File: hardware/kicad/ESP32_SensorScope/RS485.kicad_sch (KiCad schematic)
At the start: 27 parts, among them J1 RS485_A, J2 RS485_B, J3 RS485_A, J4 RS485_B, Q1 PMOS, Q2 NMOS, U3 SN74LV1T125DBV, U4 SP3481CN OR SN65HVD485E, U5 ASSR-1218

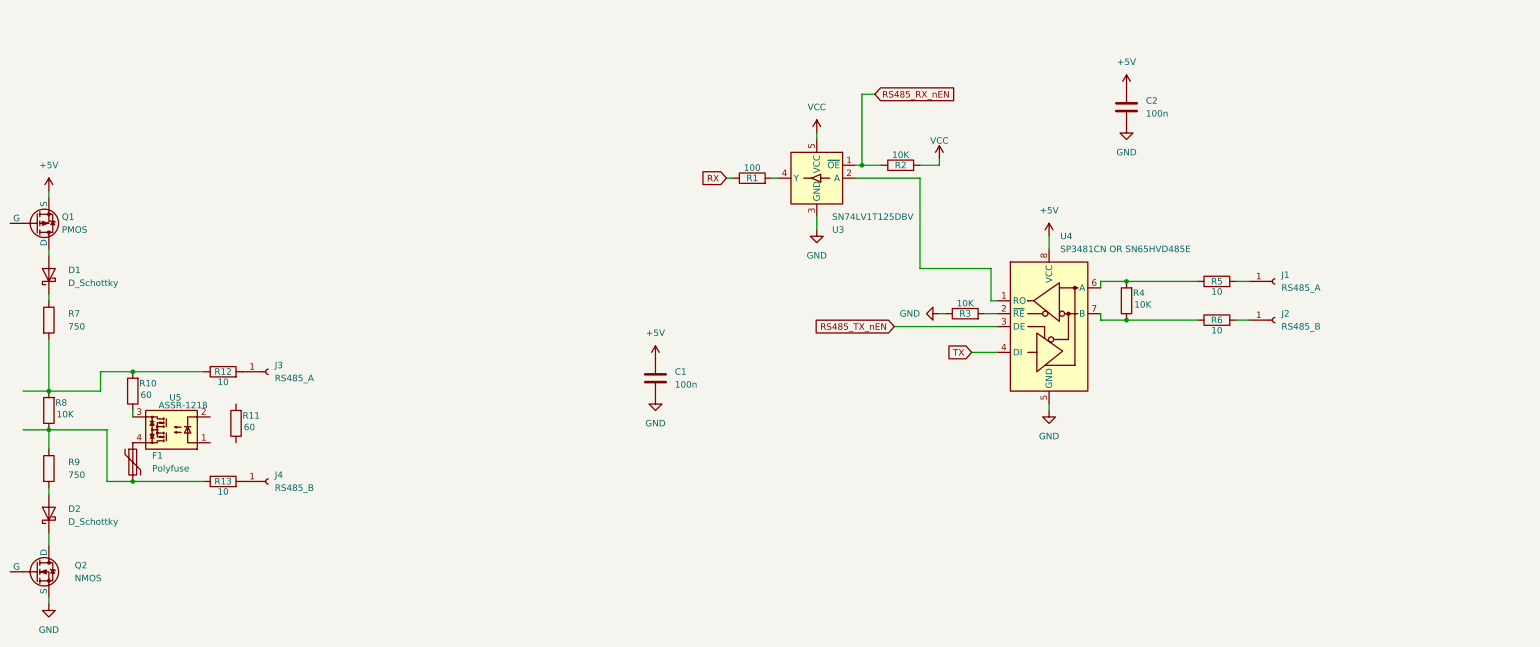
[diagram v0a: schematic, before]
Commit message: Various changes
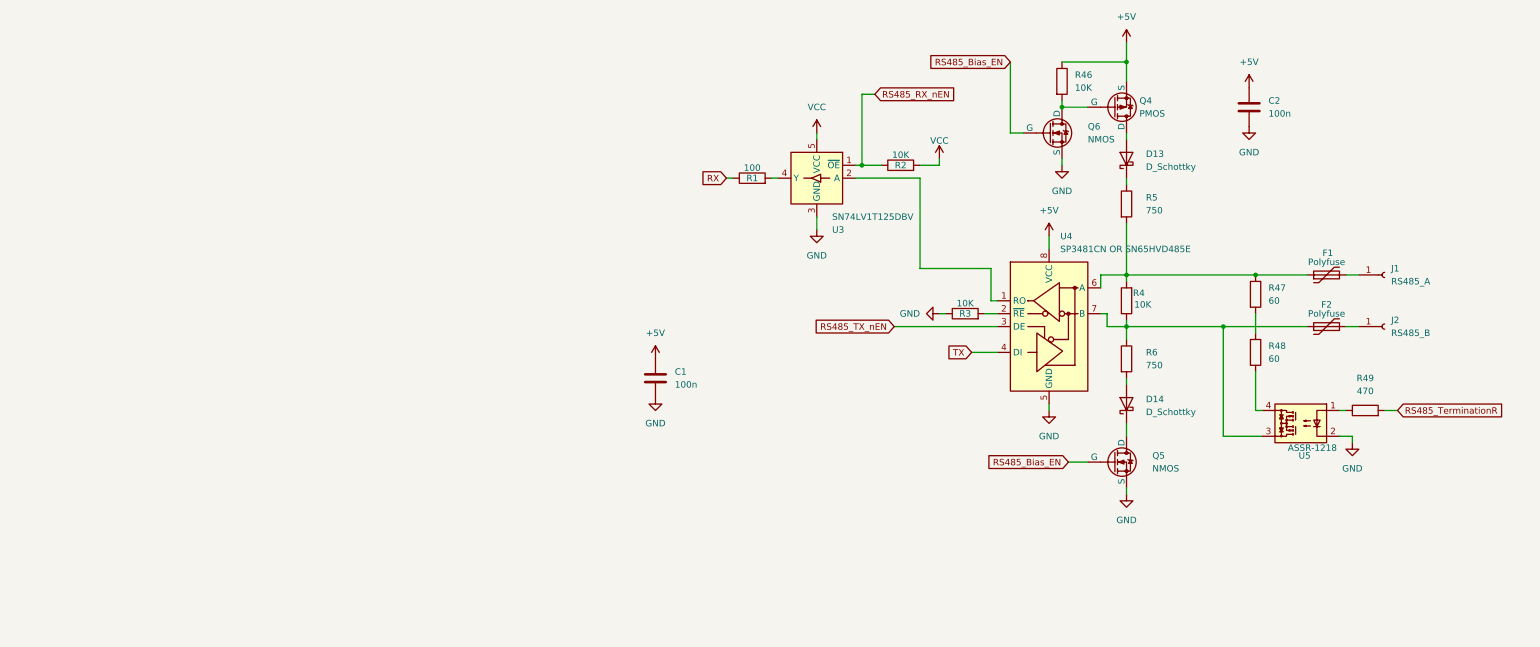
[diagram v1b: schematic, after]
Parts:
- removed D1, D2: D_Schottky, symbol Device:D_Schottky
- removed J3: RS485_A, symbol Connector:Conn_01x01_Socket
- removed J4: RS485_B, symbol Connector:Conn_01x01_Socket
- removed Q1: PMOS, symbol Simulation_SPICE:PMOS
- removed Q2: NMOS, symbol Simulation_SPICE:NMOS
- removed R10, R11: 60, symbol Device:R
- removed R12, R13: 10, symbol Device:R
- removed R7, R9: 750, symbol Device:R
- removed R8: 10K, symbol Device:R
- added D13, D14: D_Schottky, symbol Device:D_Schottky
- added F2: Polyfuse, symbol Device:Polyfuse
- added Q4: PMOS, symbol Simulation_SPICE:PMOS
- added Q5, Q6: NMOS, symbol Simulation_SPICE:NMOS
- added R46: 10K, symbol Device:R
- added R47, R48: 60, symbol Device:R
- added R49: 470, symbol Device:R
- R5, R6: value 10 -> 750
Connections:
- net +5V: now also Q4.3 (S), R46.1
- net GND: now also U5.2, Q5.3 (S), Q6.3 (S)
- net at R4.1, R6.1, U4.7 (B): now also U5.3, F2.1
- net at J2.1 (Pin_1): now also F2.2; no longer R6.2
- net at J1.1 (Pin_1): now also F1.2; no longer R5.2
- net at R4.2, U4.6 (A): now also F1.1, R5.2, R47.1; no longer R5.1
- net at U5.4: now also R48.2; no longer F1.1
- net at U5.1: now also R49.1
- new net: Q4.2 (G), Q6.1 (D), R46.2
- new net: R47.2, R48.1
- new net: D14.2 (A), R6.2
- new net: D13.2 (A), Q4.1 (D)
- new net: D14.1 (K), Q5.1 (D)
- new net: D13.1 (K), R5.1
- new net RS485_Bias_EN: Q5.2 (G), Q6.2 (G)
- new net RS485_TerminationR: R49.2
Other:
- moved on the sheet: C2, F1, J1, J2, U5
